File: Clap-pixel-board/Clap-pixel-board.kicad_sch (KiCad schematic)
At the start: 3 parts, among them J1 USB_C_Receptacle_PowerOnly_6P, U1 STM32G070CBTx

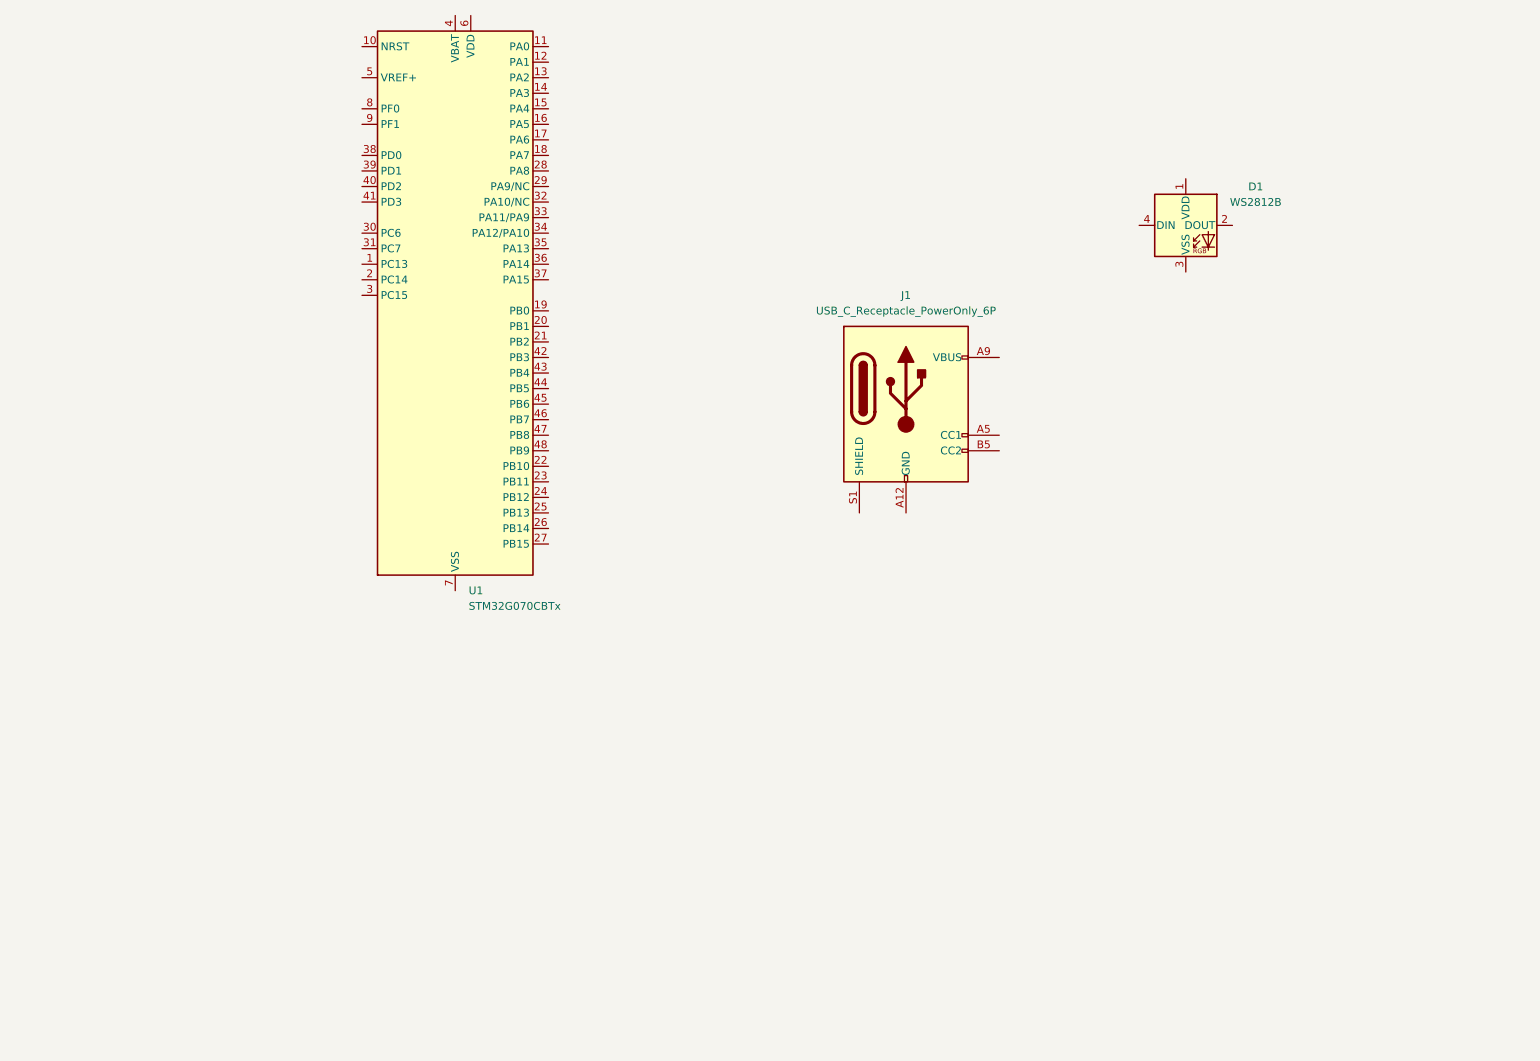
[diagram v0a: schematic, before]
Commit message: Schematic finished
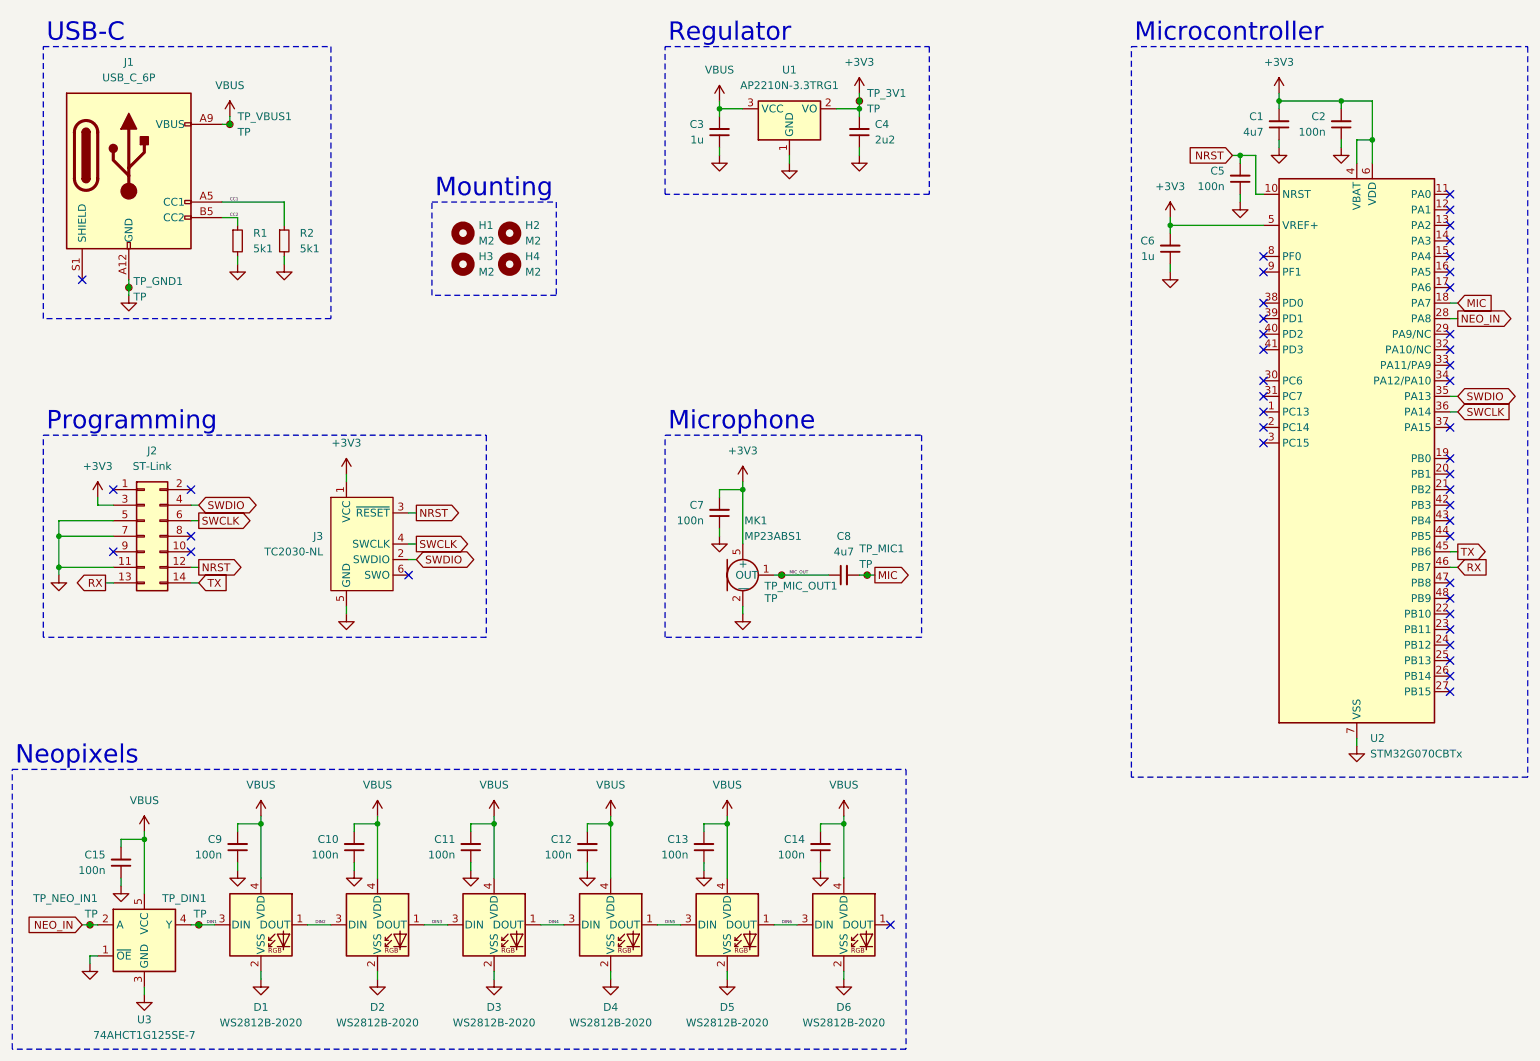
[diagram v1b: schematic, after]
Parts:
- removed D1: WS2812B, LED_SMD:LED_WS2812B_PLCC4_5.0x5.0mm_P3.2mm, symbol LED:WS2812B
- added C1, C8: 4u7, Capacitor_SMD:C_0603_1608Metric, symbol Device:C_Small
- added C10, C11, C12, C13, C14, C15, C2, C5, C7, C9: 100n, Capacitor_SMD:C_0402_1005Metric, symbol Device:C_Small
- added C3, C6: 1u, Capacitor_SMD:C_0402_1005Metric, symbol Device:C_Small
- added C4: 2u2, Capacitor_SMD:C_0603_1608Metric, symbol Device:C_Small
- added D1, D2, D3, D4, D5, D6: WS2812B-2020, LED_SMD:LED_WS2812B-2020_PLCC4_2.0x2.0mm, symbol LED:WS2812B-2020
- added H1, H2, H3, H4: M2, MountingHole:MountingHole_2.2mm_M2, symbol Mechanical:MountingHole
- added J2: ST-Link, Connector_PinHeader_1.27mm:PinHeader_2x07_P1.27mm_Vertical_SMD, symbol Connector_Generic:Conn_02x07_Odd_Even
- added J3: TC2030-NL, Connector:Tag-Connect_TC2030-IDC-NL_2x03_P1.27mm_Vertical, symbol Connector:Conn_ARM_SWD_TagConnect_TC2030-NL
- added MK1: MP23ABS1, Local_footprints:MIC_MP23ABS1TR, symbol Device:Microphone
- added R1, R2: 5k1, Resistor_SMD:R_0402_1005Metric, symbol Device:R_Small
- added TP_3V1, TP_DIN1, TP_NEO_IN1: TP, TestPoint:TestPoint_Keystone_5019_Minature, symbol Connector:TestPoint_Small
- added TP_GND1, TP_MIC1, TP_MIC_OUT1, TP_VBUS1: TP, TestPoint:TestPoint_Keystone_5015_Micro-Minature, symbol Connector:TestPoint_Small
- added U1: AP2210N-3.3TRG1, Package_TO_SOT_SMD:SOT-23-3, symbol Regulator_Linear:BD33FC0FP
- added U3: 74AHCT1G125SE-7, Package_TO_SOT_SMD:SOT-353_SC-70-5, symbol 74xGxx:NC7SZ125P5X
- J1: value USB_C_Receptacle_PowerOnly_6P -> USB_C_6P; footprint (none) -> Connector_USB:USB_C_Receptacle_GCT_USB4125-xx-x-0190_6P_TopMnt_Horizontal
- renumbered U1 to U2
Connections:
- net NRST: now reaches U2.10 (NRST)
- net NRST: now also C5.2, J2.12 (Pin_12), J3.3 (~{RESET})
- net MIC: now reaches U2.18 (PA7)
- net MIC: now also C8.2, TP_MIC1.1
- net NEO_IN: now reaches U2.28 (PA8)
- net NEO_IN: now also TP_NEO_IN1.1, U3.2 (A)
- net SWDIO: now reaches U2.35 (PA13)
- net SWDIO: now also J2.4 (Pin_4), J3.2 (SWDIO)
- net SWCLK: now reaches U2.36 (PA14)
- net SWCLK: now also J2.6 (Pin_6), J3.4 (SWCLK)
- net +3V3: now reaches U2.4 (VBAT)
- net +3V3: now also U2.5 (VREF+), U2.6 (VDD), C1.2, C2.2, C4.2, C6.2, C7.2, J2.3 (Pin_3), J3.1 (VCC), MK1.5 (+), TP_3V1.1, U1.2 (VO)
- net TX: now reaches U2.45 (PB6)
- net TX: now also J2.14 (Pin_14)
- net RX: now reaches U2.46 (PB7)
- net RX: now also J2.13 (Pin_13)
- net GND: now reaches U2.7 (VSS)
- net GND: now also J1.A12 (GND), J1.B12 (GND), C1.1, C10.1, C11.1, C12.1, C13.1, C14.1, C15.1, C2.1, C3.1, C4.1, C5.1, C6.1, C7.1, C9.1, D1.2 (VSS), D2.2 (VSS), D3.2 (VSS), D4.2 (VSS), D5.2 (VSS), D6.2 (VSS), J2.11 (Pin_11), J2.5 (Pin_5), J2.7 (Pin_7), J3.5 (GND), MK1.2 (|), MK1.3 (-), MK1.4 (-), R1.2, R2.2, TP_GND1.1, U1.1 (GND), U3.1 (~{OE}), U3.3 (GND)
- net CC1: now reaches J1.A5 (CC1)
- net CC1: now also R2.1
- net VBUS: now reaches J1.A9 (VBUS), J1.B9 (VBUS)
- net VBUS: now also C10.2, C11.2, C12.2, C13.2, C14.2, C15.2, C3.2, C9.2, D1.4 (VDD), D2.4 (VDD), D3.4 (VDD), D4.4 (VDD), D5.4 (VDD), D6.4 (VDD), TP_VBUS1.1, U1.3 (VCC), U3.5 (VCC)
- net CC2: now reaches J1.B5 (CC2)
- net CC2: now also R1.1
- new net DIN1: D1.3 (DIN), TP_DIN1.1, U3.4 (Y)
- new net DIN2: D1.1 (DOUT), D2.3 (DIN)
- new net DIN3: D2.1 (DOUT), D3.3 (DIN)
- new net DIN4: D3.1 (DOUT), D4.3 (DIN)
- new net DIN5: D4.1 (DOUT), D5.3 (DIN)
- new net DIN6: D5.1 (DOUT), D6.3 (DIN)
- new net MIC_OUT: C8.1, MK1.1 (OUT), TP_MIC_OUT1.1
- no-connect marks 0 -> 45
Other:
- note added: "Microcontroller"
- note added: "Microphone"
- note added: "Mounting"
- note added: "Neopixels"
- note added: "Programming"
- note added: "Regulator"
- note added: "USB-C"
- moved on the sheet: J1, U2
